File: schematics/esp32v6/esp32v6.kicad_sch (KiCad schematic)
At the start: 39 parts, among them J1 screen connector, J2 external connector, J3 USB_B_Micro, Q1 SS8050, Q2 SS8050, Q3 SS8050, SW1 RESET, SW2 FLASH, SW3 POWER, U1 ESP32-S, U2 IP5306, U3 AMS1117-3.3, U4 CH340C_C7464026

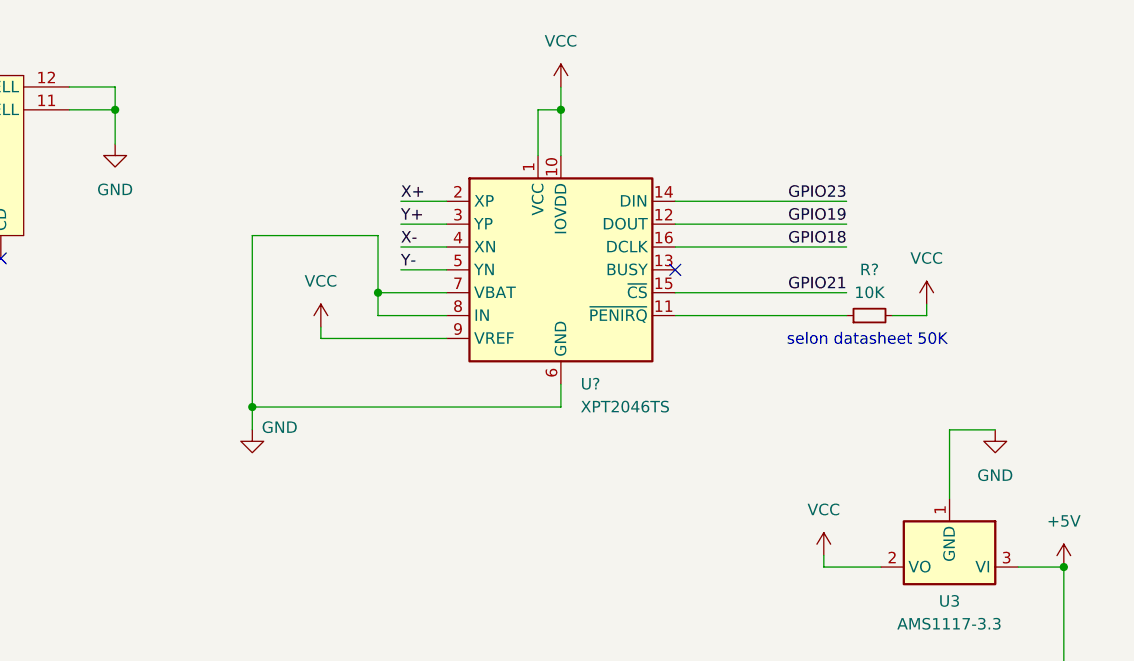
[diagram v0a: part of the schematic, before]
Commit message: Updating schematic
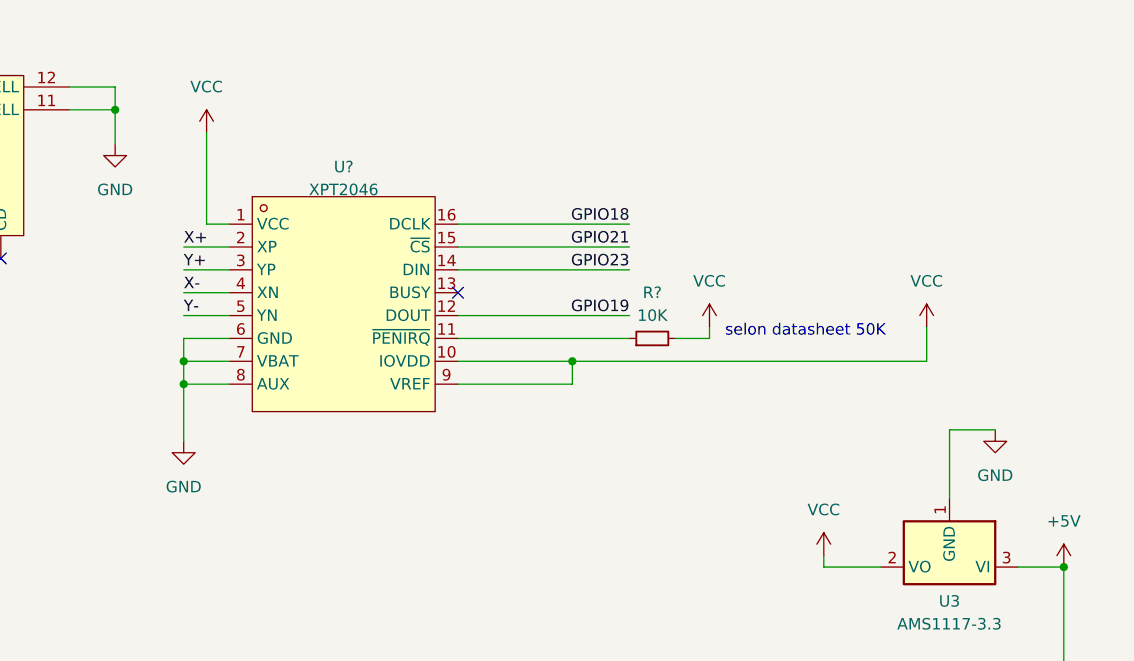
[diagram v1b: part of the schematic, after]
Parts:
- removed U?: XPT2046TS, Package_SO:TSSOP-16_4.4x5mm_P0.65mm, symbol Driver_Display:XPT2046TS
- added U?: XPT2046, LSC_Symbols:TSSOP-16_L5.0-W4.4-P0.65-LS6.4-BL, symbol LSC_Symbols:XPT2046
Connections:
- net GND: now also U?.6 (GND), U?.7 (VBAT), U?.8 (AUX)
- net GPIO18: now also U?.16 (DCLK)
- net GPIO19: now also U?.12 (DOUT)
- net GPIO21: now also U?.15 (~{CS})
- net GPIO23: now also U?.14 (DIN)
- net VCC: now also U?.1 (VCC), U?.10 (IOVDD), U?.9 (VREF)
- net X+: now also U?.2 (XP)
- net X-: now also U?.4 (XN)
- net Y+: now also U?.3 (YP)
- net Y-: now also U?.5 (YN)
- net at R?.1: now also U?.11 (~{PENIRQ})
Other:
- moved on the sheet: R?
